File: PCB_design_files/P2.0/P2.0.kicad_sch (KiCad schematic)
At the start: 40 parts, among them J1 Conn_01x02_Pin, U1 INA819IDRGR, U2 TPS60400DBVR, U3 TPS61094, U4 TC1044S, U5 NRF52832-QFAA-R

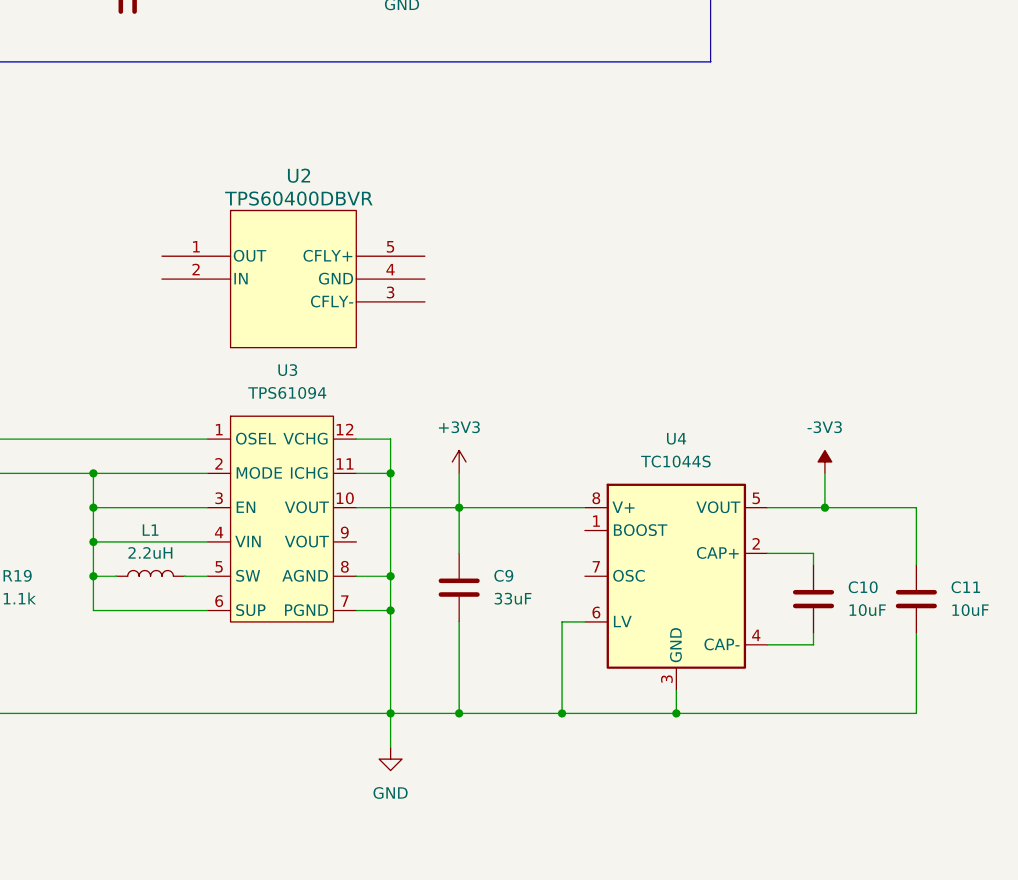
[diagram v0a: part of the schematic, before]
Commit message: Done
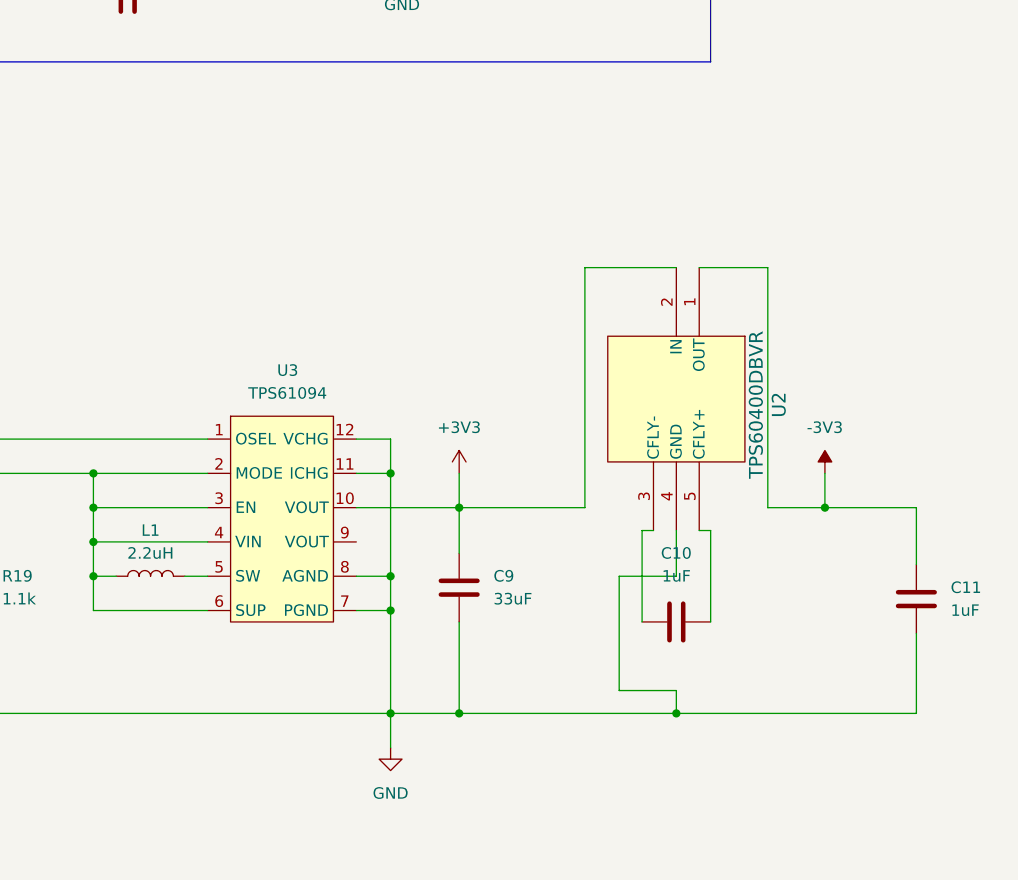
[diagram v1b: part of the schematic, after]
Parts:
- removed U4: TC1044S, Library:TC1044SEOA713, symbol Regulator_SwitchedCapacitor:LTC1044
- C10, C11: value 10uF -> 1uF
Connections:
- net +3V3: now also U2.2 (IN)
- net -3V3: now also U2.1 (OUT)
- net GND: now also U2.4 (GND)
- net at C10.1: now also U2.5 (CFLY+)
- net at C10.2: now also U2.3 (CFLY-)
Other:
- moved on the sheet: C10, U2
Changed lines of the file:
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@@
   (junction (at 212.09 161.29) (diameter 0) (color 0 0 0 0)
   )
-  (junction (at 289.56 161.29) (diameter 0) (color 0 0 0 0)
-  )
   (junction (at 271.78 71.12) (diameter 0) (color 0 0 0 0)
   )
@@
     (stroke (width 0) (type default))
   )
+  (wire (pts (xy 299.72 140.97) (xy 298.45 140.97))
+    (stroke (width 0) (type default))
+  )
   (wire (pts (xy 278.13 161.29) (xy 270.51 161.29))
     (stroke (width 0) (type default))
@@
     (stroke (width 0) (type default))
   )
+  (wire (pts (xy 295.91 158.75) (xy 302.26 158.75))
+    (stroke (width 0) (type default))
+  )
   (wire (pts (xy 66.04 43.18) (xy 66.04 40.64))
     (stroke (width 0) (type default))
@@
     (stroke (width 0) (type default))
   )
+  (wire (pts (xy 298.45 140.97) (xy 298.45 151.13))
+    (stroke (width 0) (type default))
+  )
+  (wire (pts (xy 312.42 138.43) (xy 312.42 111.76))
+    (stroke (width 0) (type default))
+  )
   (wire (pts (xy 270.51 146.05) (xy 270.51 149.86))
     (stroke (width 0) (type default))
@@
     (stroke (width 0) (type default))
   )
+  (wire (pts (xy 306.07 151.13) (xy 306.07 140.97))
+    (stroke (width 0) (type default))
+  )
   (wire (pts (xy 199.39 156.21) (xy 199.39 161.29))
     (stroke (width 0) (type default))
@@
     (stroke (width 0) (type default))
   )
-  (wire (pts (xy 278.13 161.29) (xy 289.56 161.29))
+  (wire (pts (xy 278.13 161.29) (xy 302.26 161.29))
     (stroke (width 0) (type default))
   )
@@
     (stroke (width 0) (type default))
   )
-  (wire (pts (xy 289.56 151.13) (xy 289.56 161.29))
-    (stroke (width 0) (type default))
-  )
   (wire (pts (xy 57.15 50.8) (xy 63.5 50.8))
     (stroke (width 0) (type default))
@@
     (stroke (width 0) (type default))
   )
+  (wire (pts (xy 306.07 140.97) (xy 304.8 140.97))
+    (stroke (width 0) (type default))
+  )
   (wire (pts (xy 38.1 40.64) (xy 31.75 40.64))
     (stroke (width 0) (type default))
@@
     (stroke (width 0) (type default))
   )
+  (wire (pts (xy 302.26 140.97) (xy 302.26 146.05))
+    (stroke (width 0) (type default))
+  )
   (wire (pts (xy 266.7 130.81) (xy 270.51 130.81))
     (stroke (width 0) (type default))
@@
     (stroke (width 0) (type default))
   )
+  (wire (pts (xy 295.91 146.05) (xy 295.91 158.75))
+    (stroke (width 0) (type default))
+  )
   (wire (pts (xy 237.49 138.43) (xy 237.49 142.24))
     (stroke (width 0) (type default))
@@
     (stroke (width 0) (type default))
   )
-  (wire (pts (xy 317.5 143.51) (xy 312.42 143.51))
-    (stroke (width 0) (type default))
-  )
   (wire (pts (xy 151.13 66.04) (xy 232.41 66.04))
     (stroke (width 0) (type default))
@@
     (stroke (width 0) (type default))
   )
-  (wire (pts (xy 317.5 152.4) (xy 317.5 153.67))
-    (stroke (width 0) (type default))
-  )
   (wire (pts (xy 135.89 50.8) (xy 135.89 67.31))
     (stroke (width 0) (type default))
@@
     (stroke (width 0) (type default))
   )
-  (wire (pts (xy 289.56 151.13) (xy 292.1 151.13))
-    (stroke (width 0) (type default))
-  )
   (wire (pts (xy 171.45 50.8) (xy 173.99 50.8))
     (stroke (width 0) (type default))
@@
     (stroke (width 0) (type default))
   )
-  (wire (pts (xy 302.26 161.29) (xy 289.56 161.29))
-    (stroke (width 0) (type default))
-  )
   (wire (pts (xy 189.23 151.13) (xy 189.23 161.29))
     (stroke (width 0) (type default))
@@
     (stroke (width 0) (type default))
   )
+  (wire (pts (xy 302.26 111.76) (xy 292.1 111.76))
+    (stroke (width 0) (type default))
+  )
+  (wire (pts (xy 292.1 111.76) (xy 292.1 138.43))
+    (stroke (width 0) (type default))
+  )
   (wire (pts (xy 144.78 29.21) (xy 144.78 34.29))
     (stroke (width 0) (type default))
@@
     (stroke (width 0) (type default))
   )
+  (wire (pts (xy 302.26 146.05) (xy 295.91 146.05))
+    (stroke (width 0) (type default))
+  )
   (wire (pts (xy 38.1 40.64) (xy 66.04 40.64))
     (stroke (width 0) (type default))
   )
+  (wire (pts (xy 304.8 111.76) (xy 312.42 111.76))
+    (stroke (width 0) (type default))
+  )
   (wire (pts (xy 97.79 45.72) (xy 105.41 45.72))
     (stroke (width 0) (type default))
@@
     (stroke (width 0) (type default))
   )
-  (wire (pts (xy 317.5 144.78) (xy 317.5 143.51))
-    (stroke (width 0) (type default))
-  )
   (wire (pts (xy 133.35 71.12) (xy 133.35 64.77))
     (stroke (width 0) (type default))
@@
   )
   (wire (pts (xy 318.77 134.62) (xy 318.77 138.43))
-    (stroke (width 0) (type default))
-  )
-  (wire (pts (xy 317.5 153.67) (xy 312.42 153.67))
     (stroke (width 0) (type default))
   )
@@
     )
   )
-  (symbol (lib_id "Device:C") (at 317.5 148.59 180) (unit 1)
-    (in_bom yes) (on_board yes) (dnp no) (fields_autoplaced)
-    (property "Reference" "C10" (at 321.31 147.32 0)
-      (effects (font (size 1.27 1.27)) (justify right))
-    )
-    (property "Value" "10uF" (at 321.31 149.86 0)
-      (effects (font (size 1.27 1.27)) (justify right))
-    )
-    (property "Footprint" "Capacitor_SMD:C_0805_2012Metric" (at 316.5348 144.78 0)
-      (effects (font (size 1.27 1.27)) hide)
-    )
-    (property "Datasheet" "~" (at 317.5 148.59 0)
+  (symbol (lib_id "Device:C") (at 302.26 151.13 270) (unit 1)
+    (in_bom yes) (on_board yes) (dnp no) (fields_autoplaced)
+    (property "Reference" "C10" (at 302.26 143.51 90)
+      (effects (font (size 1.27 1.27)))
+    )
+    (property "Value" "1uF" (at 302.26 146.05 90)
+      (effects (font (size 1.27 1.27)))
+    )
+    (property "Footprint" "Capacitor_SMD:C_0805_2012Metric" (at 298.45 152.0952 0)
+      (effects (font (size 1.27 1.27)) hide)
+    )
+    (property "Datasheet" "~" (at 302.26 151.13 0)
       (effects (font (size 1.27 1.27)) hide)
     )
@@
     )
   )
-  (symbol (lib_id "Regulator_SwitchedCapacitor:LTC1044") (at 302.26 146.05 0) (unit 1)
-    (in_bom yes) (on_board yes) (dnp no) (fields_autoplaced)
-    (property "Reference" "U4" (at 302.26 130.81 0)
-      (effects (font (size 1.27 1.27)))
-    )
-    (property "Value" "TC1044S" (at 302.26 133.35 0)
-      (effects (font (size 1.27 1.27)))
-    )
-    (property "Footprint" "Library:TC1044SEOA713" (at 304.8 148.59 0)
-      (effects (font (size 1.27 1.27)) hide)
-    )
-    (property "Datasheet" "" (at 304.8 148.59 0)
-      (effects (font (size 1.27 1.27)) hide)
-    )
-    (pin "1")
-    (pin "7")
-    (pin "2")
-    (pin "5")
-    (pin "4")
-    (pin "6")
-    (pin "3")
-    (pin "8")
-    (instances
-      (project "P2.0"
-        (path "/cc4d5c34-4776-48f9-a8ce-15f2c8e358ac"
-          (reference "U4") (unit 1)
-        )
-      )
-    )
-  )
   (symbol (lib_id "Device:R") (at 133.35 34.29 0) (unit 1)
     (in_bom yes) (on_board yes) (dnp no) (fields_autoplaced)
@@
       (effects (font (size 1.27 1.27)) (justify right))
     )
-    (property "Value" "10uF" (at 332.74 149.86 0)
+    (property "Value" "1uF" (at 332.74 149.86 0)
       (effects (font (size 1.27 1.27)) (justify right))
     )
@@
     )
   )
-  (symbol (lib_id "TPS60400DBVR:TPS60400DBVR") (at 252.73 105.41 0) (unit 1)
+  (symbol (lib_id "TPS60400DBVR:TPS60400DBVR") (at 309.88 119.38 270) (unit 1)
     (in_bom yes) (on_board yes) (dnp no)
-    (property "Reference" "U2" (at 260.35 101.6 0)
+    (property "Reference" "U2" (at 313.69 127 0)
       (effects (font (size 1.524 1.524)))
     )
-    (property "Value" "TPS60400DBVR" (at 260.35 104.14 0)
+    (property "Value" "TPS60400DBVR" (at 311.15 127 0)
       (effects (font (size 1.524 1.524)))
     )
-    (property "Footprint" "DBV5" (at 252.73 105.41 0)
+    (property "Footprint" "DBV5" (at 309.88 119.38 0)
       (effects (font (size 1.27 1.27) italic) hide)
     )
-    (property "Datasheet" "TPS60400DBVR" (at 252.73 105.41 0)
+    (property "Datasheet" "TPS60400DBVR" (at 309.88 119.38 0)
       (effects (font (size 1.27 1.27) italic) hide)
     )
